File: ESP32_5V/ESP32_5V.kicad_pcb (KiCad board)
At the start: 2 copper layers, 99.9 x 71.2 mm, 32 parts, among them J1 Conn_01x11, J10 Conn_01x11, J11 Conn_01x11, J12 Conn_01x11, J13 Conn_01x11, J14 Conn_01x11, J15 Conn_01x11, J16 Conn_01x11, J2 Conn_01x15, J3 Conn_01x15, J4 Conn_01x11, J5 Screw_Terminal_01x11, J6 Screw_Terminal_01x11, J7 Conn_01x11, J8 Conn_01x11, J9 Conn_01x11, U1 TXS0108EPW, U2 TXS0108EPW, U3 TXS0108EPW

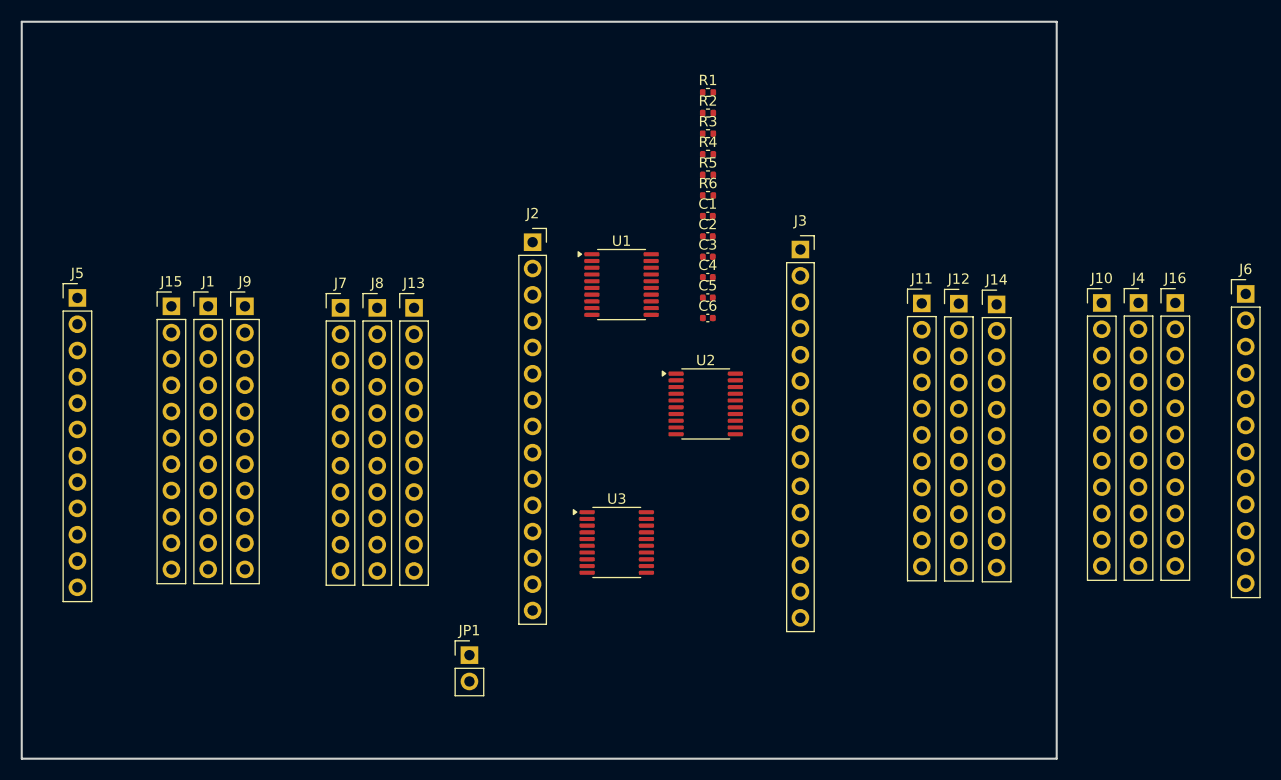
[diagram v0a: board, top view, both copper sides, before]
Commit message: update
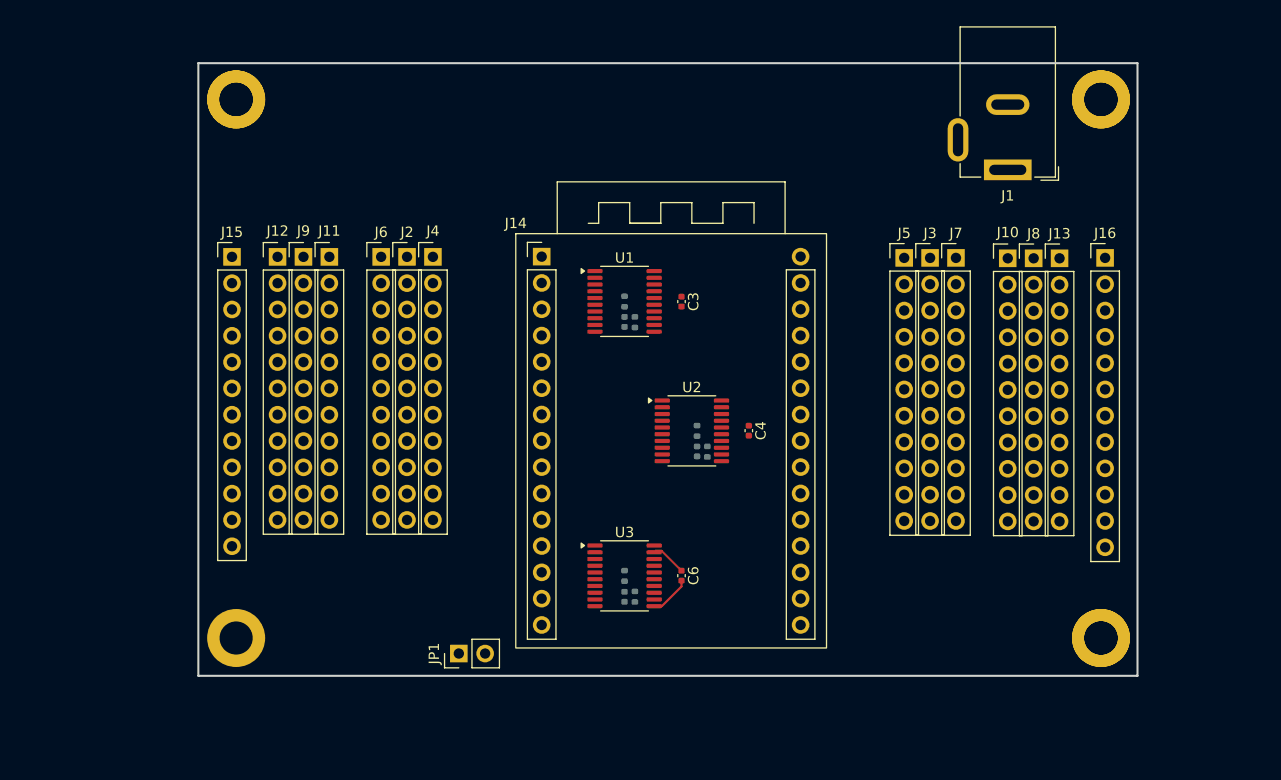
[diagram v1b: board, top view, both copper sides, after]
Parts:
- added ?: , , F.Cu at (146.0, 36.0)
- added ?: , , F.Cu at (62.5, 36.0)
- added ?: , , F.Cu at (146.0, 88.0)
- added REF**: MountingHole_3.2mm_M3_DIN965_Pad, MountingHole:MountingHole_3.2mm_M3_DIN965_Pad, F.Cu at (146.0, 88.0)
- added REF**: MountingHole_3.2mm_M3_DIN965_Pad, MountingHole:MountingHole_3.2mm_M3_DIN965_Pad, F.Cu at (62.5, 36.0)
- added REF**: MountingHole_3.2mm_M3_DIN965_Pad, MountingHole:MountingHole_3.2mm_M3_DIN965_Pad, F.Cu at (62.5, 88.0)
- added REF**: MountingHole_3.2mm_M3_DIN965_Pad, MountingHole:MountingHole_3.2mm_M3_DIN965_Pad, F.Cu at (146.0, 36.0)
- C1, C2, C5, R1, R4, R5, R6: moved to B.Cu
- J1: value Conn_01x11 -> Jack-DC; footprint Connector_PinHeader_2.54mm:PinHeader_1x11_P2.54mm_Vertical -> Connector_BarrelJack:BarrelJack_GCT_DCJ200-10-A_Horizontal
- J14: value Conn_01x11 -> ~; footprint Connector_PinHeader_2.54mm:PinHeader_1x11_P2.54mm_Vertical -> ESP32_5V:ESP32_dispositivo
- J15, J16: value Conn_01x11 -> Screw_Terminal_01x11; footprint Connector_PinHeader_2.54mm:PinHeader_1x11_P2.54mm_Vertical -> Connector_PinHeader_2.54mm:PinHeader_1x12_P2.54mm_Vertical
- J2, J3: value Conn_01x15 -> Conn_01x11; footprint Connector_PinSocket_2.54mm:PinSocket_1x15_P2.54mm_Vertical -> Connector_PinHeader_2.54mm:PinHeader_1x11_P2.54mm_Vertical
- J5, J6: value Screw_Terminal_01x11 -> Conn_01x11; footprint Connector_PinHeader_2.54mm:PinHeader_1x12_P2.54mm_Vertical -> Connector_PinHeader_2.54mm:PinHeader_1x11_P2.54mm_Vertical
- R2: value 0 -> 10k; moved to B.Cu
- R3: value 10k -> 0; moved to B.Cu
- moved J6 83.6 mm to (76.5, 51.2)
- moved J5 79.9 mm to (127.0, 51.3)
- moved J1 78.3 mm to (137.0, 42.8), turned to 180 degrees
- moved J4 68.3 mm to (81.5, 51.2)
- moved J12 65.9 mm to (66.5, 51.2)
- moved J8 63.6 mm to (139.5, 51.3)
- moved J13 62.5 mm to (142.0, 51.3)
- moved J7 59.6 mm to (132.0, 51.3)
- moved J11 57.4 mm to (71.5, 51.2)
- moved R5 39.5 mm to (100.0, 82.0), turned to 90 degrees
- moved R6 39.4 mm to (101.0, 84.0), turned to 90 degrees
- moved J14 34.1 mm to (104.5, 69.0)
- moved R2 30.7 mm to (107.0, 68.0), turned to -90 degrees
- moved C5 30.0 mm to (100.0, 84.0), turned to -90 degrees
- moved R4 28.7 mm to (108.0, 70.0), turned to 90 degrees
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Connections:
- C1 pad 1: +5V -> +3V3
- C3 pad 1: +3V3 -> +5V
- J1 pad 1: +5V -> VCC
- J1 pad 2: +5V -> GND
- J1 pad 3: +5V -> (no net)
- J12 pad 1: +3V3 -> /Conector_5V/D34_5V
- J12 pad 10: +3V3 -> /Conector_5V/D13_5V
- J12 pad 11: +3V3 -> /Conector_5V/D23_5V
- J12 pad 2: +3V3 -> /Conector_5V/D35_5V
- J12 pad 3: +3V3 -> /Conector_5V/D32_5V
- J12 pad 4: +3V3 -> /Conector_5V/D33_5V
- J12 pad 5: +3V3 -> /Conector_5V/D25_5V
- J12 pad 6: +3V3 -> /Conector_5V/D26_5V
- J12 pad 7: +3V3 -> /Conector_5V/D27_5V
- J12 pad 8: +3V3 -> /Conector_5V/D14_5V
- J12 pad 9: +3V3 -> /Conector_5V/D12_5V
- J13 pad 1: GND -> /Conector_5V/D22_5V
- J13 pad 10: GND -> /Conector_5V/D15_5V
- J13 pad 11: GND -> unconnected-(J13-Pin_11-Pad11)
- J13 pad 2: GND -> /Conector_5V/D21_5V
- J13 pad 3: GND -> /Conector_5V/D19_5V
- J13 pad 4: GND -> /Conector_5V/D18_5V
- J13 pad 5: GND -> /Conector_5V/D5_5V
- J13 pad 6: GND -> /Conector_5V/D17_5V
- J13 pad 7: GND -> /Conector_5V/D16_5V
- J13 pad 8: GND -> /Conector_5V/D4_5V
- J13 pad 9: GND -> /Conector_5V/D2_5V
- J14 pad 1: /Conector_3V3/D12 -> unconnected-(J14-Pad1)
- J14 pad 10: /Conector_3V3/D16 -> /Conector_3V3/D27
- J14 pad 11: /Conector_3V3/D4 -> /Conector_3V3/D14
- J14 pad 2: /Conector_3V3/D13 -> unconnected-(J14-Pad2)
- J14 pad 3: /Conector_3V3/D23 -> unconnected-(J14-Pad3)
- J14 pad 4: /Conector_3V3/D22 -> /Conector_3V3/D34
- J14 pad 5: /Conector_3V3/D21 -> /Conector_3V3/D35
- J14 pad 6: /Conector_3V3/D19 -> /Conector_3V3/D32
- J14 pad 7: /Conector_3V3/D18 -> /Conector_3V3/D33
- J14 pad 8: /Conector_3V3/D5 -> /Conector_3V3/D25
- J14 pad 9: /Conector_3V3/D17 -> /Conector_3V3/D26
- J2 pad 1: unconnected-(J2-Pin_1-Pad1) -> +3V3
- J2 pad 10: /Conector_3V3/D27 -> +3V3
- J2 pad 11: /Conector_3V3/D14 -> +3V3
- J2 pad 2: unconnected-(J2-Pin_2-Pad2) -> +3V3
- J2 pad 3: unconnected-(J2-Pin_3-Pad3) -> +3V3
- J2 pad 4: /Conector_3V3/D34 -> +3V3
- J2 pad 5: /Conector_3V3/D35 -> +3V3
- J2 pad 6: /Conector_3V3/D32 -> +3V3
- J2 pad 7: /Conector_3V3/D33 -> +3V3
- J2 pad 8: /Conector_3V3/D25 -> +3V3
- J2 pad 9: /Conector_3V3/D26 -> +3V3
- J3 pad 1: /ESP32/D23 -> +3V3
- J3 pad 10: /ESP32/D16 -> +3V3
- J3 pad 11: /ESP32/D4 -> +3V3
- J3 pad 2: /ESP32/D22 -> +3V3
- J3 pad 3: unconnected-(J3-Pin_3-Pad3) -> +3V3
- J3 pad 4: unconnected-(J3-Pin_4-Pad4) -> +3V3
- J3 pad 5: /ESP32/D21 -> +3V3
- J3 pad 6: /ESP32/D19 -> +3V3
- J3 pad 7: /ESP32/D18 -> +3V3
- J3 pad 8: /ESP32/D5 -> +3V3
- J3 pad 9: /ESP32/D17 -> +3V3
- J4 pad 1: +5V -> GND
- J4 pad 10: +5V -> GND
- J4 pad 11: +5V -> GND
- J4 pad 2: +5V -> GND
- J4 pad 3: +5V -> GND
- J4 pad 4: +5V -> GND
- J4 pad 5: +5V -> GND
- J4 pad 6: +5V -> GND
- J4 pad 7: +5V -> GND
- J4 pad 8: +5V -> GND
- J4 pad 9: +5V -> GND
- J5 pad 1: /conector_atornillado/D34_5V -> GND
- J5 pad 10: /conector_atornillado/D13_5V -> GND
- J5 pad 11: /conector_atornillado/D23_5V -> GND
- J5 pad 2: /conector_atornillado/D35_5V -> GND
- J5 pad 3: /conector_atornillado/D32_5V -> GND
- J5 pad 4: /conector_atornillado/D33_5V -> GND
- J5 pad 5: /conector_atornillado/D25_5V -> GND
- J5 pad 6: /conector_atornillado/D26_5V -> GND
- J5 pad 7: /conector_atornillado/D27_5V -> GND
- J5 pad 8: /conector_atornillado/D14_5V -> GND
- J5 pad 9: /conector_atornillado/D12_5V -> GND
- J6 pad 1: /conector_atornillado/D22_5V -> /Conector_3V3/D34
- J6 pad 10: /conector_atornillado/D15_5V -> /Conector_3V3/D13
- J6 pad 2: /conector_atornillado/D21_5V -> /Conector_3V3/D35
- J6 pad 3: /conector_atornillado/D19_5V -> /Conector_3V3/D32
- J6 pad 4: /conector_atornillado/D18_5V -> /Conector_3V3/D33
- J6 pad 5: /conector_atornillado/D5_5V -> /Conector_3V3/D25
- J6 pad 6: /conector_atornillado/D17_5V -> /Conector_3V3/D26
- J6 pad 7: /conector_atornillado/D16_5V -> /Conector_3V3/D27
- J6 pad 8: /conector_atornillado/D4_5V -> /Conector_3V3/D14
- J6 pad 9: /conector_atornillado/D2_5V -> /Conector_3V3/D12
- J7 pad 1: /Conector_3V3/D34 -> /Conector_3V3/D12
- J7 pad 10: /Conector_3V3/D13 -> /Conector_3V3/D16
- J7 pad 11: unconnected-(J7-Pin_11-Pad11) -> /Conector_3V3/D4
- J7 pad 2: /Conector_3V3/D35 -> /Conector_3V3/D13
- J7 pad 3: /Conector_3V3/D32 -> /Conector_3V3/D23
- J7 pad 4: /Conector_3V3/D33 -> /Conector_3V3/D22
- J7 pad 5: /Conector_3V3/D25 -> /Conector_3V3/D21
- J7 pad 6: /Conector_3V3/D26 -> /Conector_3V3/D19
- J7 pad 7: /Conector_3V3/D27 -> /Conector_3V3/D18
- J7 pad 8: /Conector_3V3/D14 -> /Conector_3V3/D5
- J7 pad 9: /Conector_3V3/D12 -> /Conector_3V3/D17
- J8 pad 1: +3V3 -> +5V
- J8 pad 10: +3V3 -> +5V
- J8 pad 11: +3V3 -> +5V
- J8 pad 2: +3V3 -> +5V
- J8 pad 3: +3V3 -> +5V
- J8 pad 4: +3V3 -> +5V
- J8 pad 5: +3V3 -> +5V
- J8 pad 6: +3V3 -> +5V
- J8 pad 7: +3V3 -> +5V
- J8 pad 8: +3V3 -> +5V
- J8 pad 9: +3V3 -> +5V
- J9 pad 1: GND -> +5V
- J9 pad 10: GND -> +5V
- J9 pad 11: GND -> +5V
- J9 pad 2: GND -> +5V
- J9 pad 3: GND -> +5V
- J9 pad 4: GND -> +5V
- J9 pad 5: GND -> +5V
- J9 pad 6: GND -> +5V
- J9 pad 7: GND -> +5V
- J9 pad 8: GND -> +5V
- J9 pad 9: GND -> +5V
- JP1 pad 1: Net-(J2-Pin_15) -> Net-(JP1-A)
- R2 pad 1: Net-(U1-OE) -> GND
- R2 pad 2: +3V3 -> Net-(U2-OE)
- R3 pad 1: GND -> Net-(U1-OE)
- R3 pad 2: Net-(U2-OE) -> +3V3
- U1 pad 1: /Conector_5V/D34 -> /Conector_3V3/D34
- U1 pad 3: /Conector_5V/D35 -> /Conector_3V3/D35
- U1 pad 4: /Conector_5V/D32 -> /Conector_3V3/D32
- U1 pad 5: /Conector_5V/D33 -> /Conector_3V3/D33
- U1 pad 6: /Conector_5V/D25 -> /Conector_3V3/D25
- U1 pad 7: /Conector_5V/D26 -> /Conector_3V3/D26
- U1 pad 8: /Conector_5V/D27 -> /Conector_3V3/D27
- U1 pad 9: /Conector_5V/D14 -> /Conector_3V3/D14
- U2 pad 1: /Conector_5V/D12 -> /Conector_3V3/D12
- U2 pad 3: /Conector_5V/D13 -> /Conector_3V3/D13
- U2 pad 4: /Conector_5V/D23 -> /Conector_3V3/D23
- U2 pad 5: /Conector_5V/D22 -> /Conector_3V3/D22
- U2 pad 6: /Conector_5V/D21 -> /Conector_3V3/D21
- U2 pad 7: /Conector_5V/D19 -> /Conector_3V3/D19
- U2 pad 8: /Conector_5V/D18 -> /Conector_3V3/D18
- U2 pad 9: /Conector_5V/D5 -> /Conector_3V3/D5
- U3 pad 1: /Conector_5V/D17 -> /Conector_3V3/D17
- U3 pad 3: /Conector_5V/D16 -> /Conector_3V3/D16
- U3 pad 4: /Conector_5V/D4 -> /Conector_3V3/D4
- U3 pad 5: /Conector_5V/D2 -> /Conector_3V3/D2
- U3 pad 6: /Conector_5V/D15 -> /Conector_3V3/D15
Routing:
- net GND: track 0.00 -> 3.99 mm
- net +5V: track 0.00 -> 3.50 mm
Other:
- board size 99.9 x 71.2 mm -> 90.7 x 59.2 mm
- copper layers 2 -> 4

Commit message: update
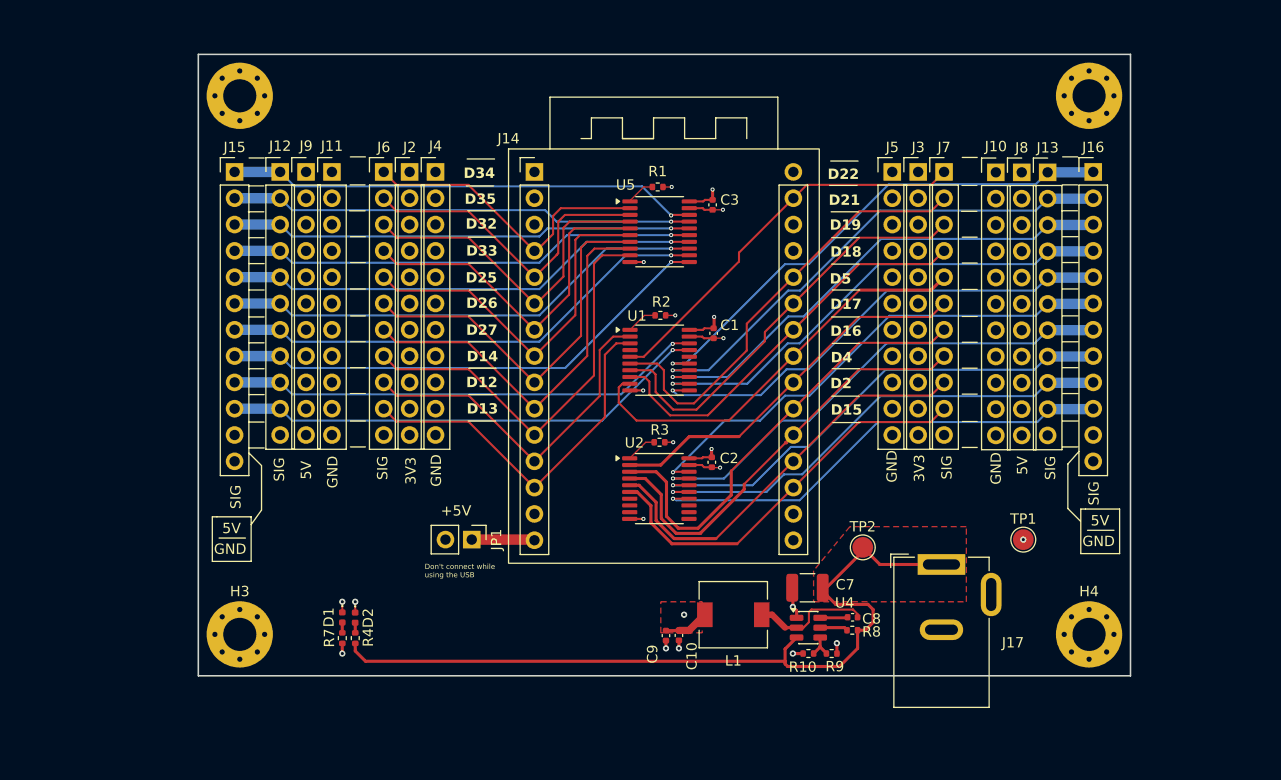
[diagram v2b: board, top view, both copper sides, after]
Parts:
- removed ? (x3): , 
- removed C4, C5, C6: 10nF, Capacitor_SMD:C_0402_1005Metric
- removed J1: Jack-DC, Connector_BarrelJack:BarrelJack_GCT_DCJ200-10-A_Horizontal
- removed R5: 10k, Resistor_SMD:R_0402_1005Metric
- removed R6: 0, Resistor_SMD:R_0402_1005Metric
- removed the REF** at (146.0, 88.0)
- removed the REF** at (62.5, 36.0)
- removed the REF** at (62.5, 88.0)
- removed the REF** at (146.0, 36.0)
- removed U3: TXS0108EPW, Package_SO:TSSOP-20_4.4x6.5mm_P0.65mm
- added C10: 10u, Capacitor_SMD:C_0402_1005Metric, F.Cu at (105.2, 87.8)
- added C7: 10u, Capacitor_SMD:C_1210_3225Metric, F.Cu at (117.7, 83.2)
- added C8: 100nF, Capacitor_SMD:C_0402_1005Metric, F.Cu at (122.0, 86.0)
- added C9: 10u, Capacitor_SMD:C_0402_1005Metric, F.Cu at (104.0, 87.8)
- added D1: LED, LED_SMD:LED_0402_1005Metric, F.Cu at (72.8, 86.0)
- added D2: LED, LED_SMD:LED_0402_1005Metric, F.Cu at (74.0, 86.0)
- added H1: MountingHole_Pad, MountingHole:MountingHole_3.2mm_M3_Pad_Via, F.Cu at (62.9, 35.6)
- added H2: MountingHole_Pad, MountingHole:MountingHole_3.2mm_M3_Pad_Via, F.Cu at (144.8, 35.6)
- added H3: MountingHole_Pad, MountingHole:MountingHole_3.2mm_M3_Pad_Via, F.Cu at (62.9, 87.7)
- added H4: MountingHole_Pad, MountingHole:MountingHole_3.2mm_M3_Pad_Via, F.Cu at (144.8, 87.7)
- added J17: Barrel_Jack_MountingPin, Connector_BarrelJack:BarrelJack_GCT_DCJ200-10-A_Horizontal, F.Cu at (130.6, 80.9)
- added L1: 4,7uH, Inductor_SMD:L_6.3x6.3_H3, F.Cu at (110.5, 85.8)
- added R10: 20k, Resistor_SMD:R_0402_1005Metric, F.Cu at (117.8, 89.5)
- added R7: 10k, Resistor_SMD:R_0402_1005Metric, F.Cu at (72.8, 88.0)
- added R8: 10k, Resistor_SMD:R_0402_1005Metric, F.Cu at (122.0, 87.2)
- added R9: 110k, Resistor_SMD:R_0402_1005Metric, F.Cu at (120.0, 89.5)
- added REF**: ESD-Logo_8.9x8mm_SilkScreen, Symbol:ESD-Logo_8.9x8mm_SilkScreen, B.Cu at (104.5, 73.1)
- added REF**: OSHW-Symbol_8.9x8mm_SilkScreen, Symbol:OSHW-Symbol_8.9x8mm_SilkScreen, B.Cu at (104.0, 62.0)
- added REF**: KiCad-Logo2_8mm_SilkScreen, Symbol:KiCad-Logo2_8mm_SilkScreen, B.Cu at (103.7, 49.1)
- added TP1: TestPoint, TestPoint:TestPoint_Pad_D2.0mm, F.Cu at (138.5, 78.5)
- added TP2: TestPoint, TestPoint:TestPoint_Pad_D2.0mm, F.Cu at (123.0, 79.2)
- added U4: TPS563201, Package_TO_SOT_SMD:SOT-23-6, F.Cu at (117.8, 87.0)
- added U5: SN74LVC245APW, Package_SO:TSSOP-20_4.4x6.5mm_P0.65mm, F.Cu at (103.4, 48.8)
- C1, C2, R3: moved to F.Cu
- R1, R2: value 10k -> 0; moved to F.Cu
- R4: value 0 -> 10k; moved to F.Cu
- U1, U2: value TXS0108EPW -> SN74LVC245APW
- moved R4 38.5 mm to (74.0, 88.0)
- moved R3 11.8 mm to (103.4, 69.1), turned to 0 degrees
- moved R2 11.7 mm to (103.5, 56.9), turned to 0 degrees
- moved R1 11.5 mm to (103.2, 44.5), turned to 0 degrees
- moved JP1 11.1 mm to (85.2, 78.5), turned to -90 degrees
- moved C3 9.81 mm to (108.5, 46.2)
- moved C1 8.67 mm to (108.6, 58.6)
- moved J10 8.38 mm to (135.8, 43.0)
- moved J13 8.38 mm to (140.8, 43.0)
- moved J8 8.38 mm to (138.3, 43.0)
- moved J16 8.38 mm to (145.2, 43.0)
- moved J3 8.38 mm to (128.3, 43.0)
- moved J5 8.38 mm to (125.8, 43.0)
- moved J7 8.38 mm to (130.8, 43.0)
- moved J14 8.21 mm to (103.8, 60.8)
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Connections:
- C1 pad 1: +3V3 -> +5V
- C2 pad 1: +3V3 -> +5V
- J12 pad 11: /Conector_5V/D23_5V -> unconnected-(J12-Pin_11-Pad11)
- J14 pad 16: /Conector_3V3/D23 -> unconnected-(J14-Pad16)
- J14 pad 30: unconnected-(J14-Pad30) -> +3V3
- J15 pad 11: /Conector_5V/D23_5V -> +5V
- J15 pad 12: (no net) -> GND
- J16 pad 11: unconnected-(J16-Pin_11-Pad11) -> +5V
- J16 pad 12: (no net) -> GND
- J7 pad 1: /Conector_3V3/D12 -> /Conector_3V3/D22
- J7 pad 10: /Conector_3V3/D16 -> /Conector_3V3/D15
- J7 pad 11: /Conector_3V3/D4 -> unconnected-(J7-Pin_11-Pad11)
- J7 pad 2: /Conector_3V3/D13 -> /Conector_3V3/D21
- J7 pad 3: /Conector_3V3/D23 -> /Conector_3V3/D19
- J7 pad 4: /Conector_3V3/D22 -> /Conector_3V3/D18
- J7 pad 5: /Conector_3V3/D21 -> /Conector_3V3/D5
- J7 pad 6: /Conector_3V3/D19 -> /Conector_3V3/D17
- J7 pad 7: /Conector_3V3/D18 -> /Conector_3V3/D16
- J7 pad 8: /Conector_3V3/D5 -> /Conector_3V3/D4
- J7 pad 9: /Conector_3V3/D17 -> /Conector_3V3/D2
- R1 pad 1: GND -> Net-(U5-DIR)
- R1 pad 2: Net-(U1-OE) -> +5V
- R2 pad 1: GND -> Net-(U1-DIR)
- R2 pad 2: Net-(U2-OE) -> +5V
- R3 pad 1: Net-(U1-OE) -> Net-(U2-DIR)
- R3 pad 2: +3V3 -> +5V
- R4 pad 1: Net-(U2-OE) -> VCC
- R4 pad 2: +3V3 -> Net-(D2-A)
- U1 pad 1: /Conector_3V3/D34 -> Net-(U1-DIR)
- U1 pad 10: Net-(U1-OE) -> GND
- U1 pad 11: GND -> /Conector_5V/D5_5V
- U1 pad 12: /Conector_5V/D14_5V -> /Conector_5V/D18_5V
- U1 pad 13: /Conector_5V/D27_5V -> /Conector_5V/D19_5V
- U1 pad 14: /Conector_5V/D26_5V -> /Conector_5V/D21_5V
- U1 pad 15: /Conector_5V/D25_5V -> /Conector_5V/D22_5V
- U1 pad 16: /Conector_5V/D33_5V -> unconnected-(U1-B3-Pad16)
- U1 pad 17: /Conector_5V/D32_5V -> /Conector_5V/D13_5V
- U1 pad 18: /Conector_5V/D35_5V -> /Conector_5V/D12_5V
- U1 pad 19: +5V -> GND
- U1 pad 2: Net-(U1-OE) -> /Conector_3V3/D12
- U1 pad 20: /Conector_5V/D34_5V -> +5V
- U1 pad 3: /Conector_3V3/D35 -> /Conector_3V3/D13
- U1 pad 4: /Conector_3V3/D32 -> unconnected-(U1-A3-Pad4)
- U1 pad 5: /Conector_3V3/D33 -> /Conector_3V3/D22
- U1 pad 6: /Conector_3V3/D25 -> /Conector_3V3/D21
- U1 pad 7: /Conector_3V3/D26 -> /Conector_3V3/D19
- U1 pad 8: /Conector_3V3/D27 -> /Conector_3V3/D18
- U1 pad 9: /Conector_3V3/D14 -> /Conector_3V3/D5
- U2 pad 1: /Conector_3V3/D12 -> Net-(U2-DIR)
- U2 pad 10: Net-(U2-OE) -> GND
- U2 pad 11: GND -> unconnected-(U2-B8-Pad11)
- U2 pad 12: /Conector_5V/D5_5V -> unconnected-(U2-B7-Pad12)
- U2 pad 13: /Conector_5V/D18_5V -> unconnected-(U2-B6-Pad13)
- U2 pad 14: /Conector_5V/D19_5V -> /Conector_5V/D15_5V
- U2 pad 15: /Conector_5V/D21_5V -> /Conector_5V/D2_5V
- U2 pad 16: /Conector_5V/D22_5V -> /Conector_5V/D4_5V
- U2 pad 17: /Conector_5V/D23_5V -> /Conector_5V/D16_5V
- U2 pad 18: /Conector_5V/D13_5V -> /Conector_5V/D17_5V
- U2 pad 19: +5V -> GND
- U2 pad 2: Net-(U2-OE) -> /Conector_3V3/D17
- U2 pad 20: /Conector_5V/D12_5V -> +5V
- U2 pad 3: /Conector_3V3/D13 -> /Conector_3V3/D16
- U2 pad 4: /Conector_3V3/D23 -> /Conector_3V3/D4
- U2 pad 5: /Conector_3V3/D22 -> /Conector_3V3/D2
- U2 pad 6: /Conector_3V3/D21 -> /Conector_3V3/D15
- U2 pad 7: /Conector_3V3/D19 -> unconnected-(U2-A6-Pad7)
- U2 pad 8: /Conector_3V3/D18 -> unconnected-(U2-A7-Pad8)
- U2 pad 9: /Conector_3V3/D5 -> unconnected-(U2-A8-Pad9)
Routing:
- net +3V3: track 0.00 -> 110.6 mm
- net VCC: track 0.00 -> 78.0 mm
- net /Conector_5V/D22_5V: track 0.00 -> 49.9 mm, vias 0 -> 1
- net /Conector_5V/D21_5V: track 0.00 -> 49.1 mm, vias 0 -> 1
- net /Conector_5V/D17_5V: track 0.00 -> 49.0 mm, vias 0 -> 1
- net /Conector_5V/D14_5V: track 0.00 -> 48.6 mm, vias 0 -> 1
- net /Conector_5V/D19_5V: track 0.00 -> 48.4 mm, vias 0 -> 1
- net /Conector_5V/D16_5V: track 0.00 -> 48.1 mm, vias 0 -> 1
- net /Conector_5V/D27_5V: track 0.00 -> 47.8 mm, vias 0 -> 1
- net /Conector_5V/D18_5V: track 0.00 -> 47.6 mm, vias 0 -> 1
- net /Conector_5V/D4_5V: track 0.00 -> 47.3 mm, vias 0 -> 1
- net /Conector_5V/D13_5V: track 0.00 -> 47.2 mm, vias 0 -> 1
- net /Conector_5V/D5_5V: track 0.00 -> 47.2 mm, vias 0 -> 1
- net /Conector_5V/D26_5V: track 0.00 -> 47.0 mm, vias 0 -> 1
- net /Conector_5V/D2_5V: track 0.00 -> 46.6 mm, vias 0 -> 1
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- added copper zone on F.Cu, net +5V
- added copper zone on In2.Cu, net +5V
- added copper zone on In1.Cu, net GND
- added copper zone on F.Cu, net VCC
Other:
- board size 90.7 x 59.2 mm -> 90 x 60 mm
- board text added: "+5V"
- board text added: "3V3"
- board text added: "5V"
- board text added: "D12"
- board text added: "D13"
- board text added: "D14"
- board text added: "D15"
- board text added: "D16"
- board text added: "D17"
- board text added: "D18"
- board text added: "D19"
- board text added: "D2"
- board text added: "D21"
- board text added: "D22"
- board text added: "D25"
- board text added: "D26"
- board text added: "D27"
- board text added: "D32"
- board text added: "D33"
- board text added: "D34"
- board text added: "D35"
- board text added: "D4"
- board text added: "D5"
- board text added: "Don't connect while using the USB"
- board text added: "GND"
- board text added: "SIG"
